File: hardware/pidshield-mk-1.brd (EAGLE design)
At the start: 43 x 52 mm, 32 parts, among them IC1 MAX31855, IC2 LM2931-3.3V, Q1 2N7000, Q2 2N7000, Q3 2N7000, Q4 2N7000, U1 ARDUINO_SHIELDINSIDER

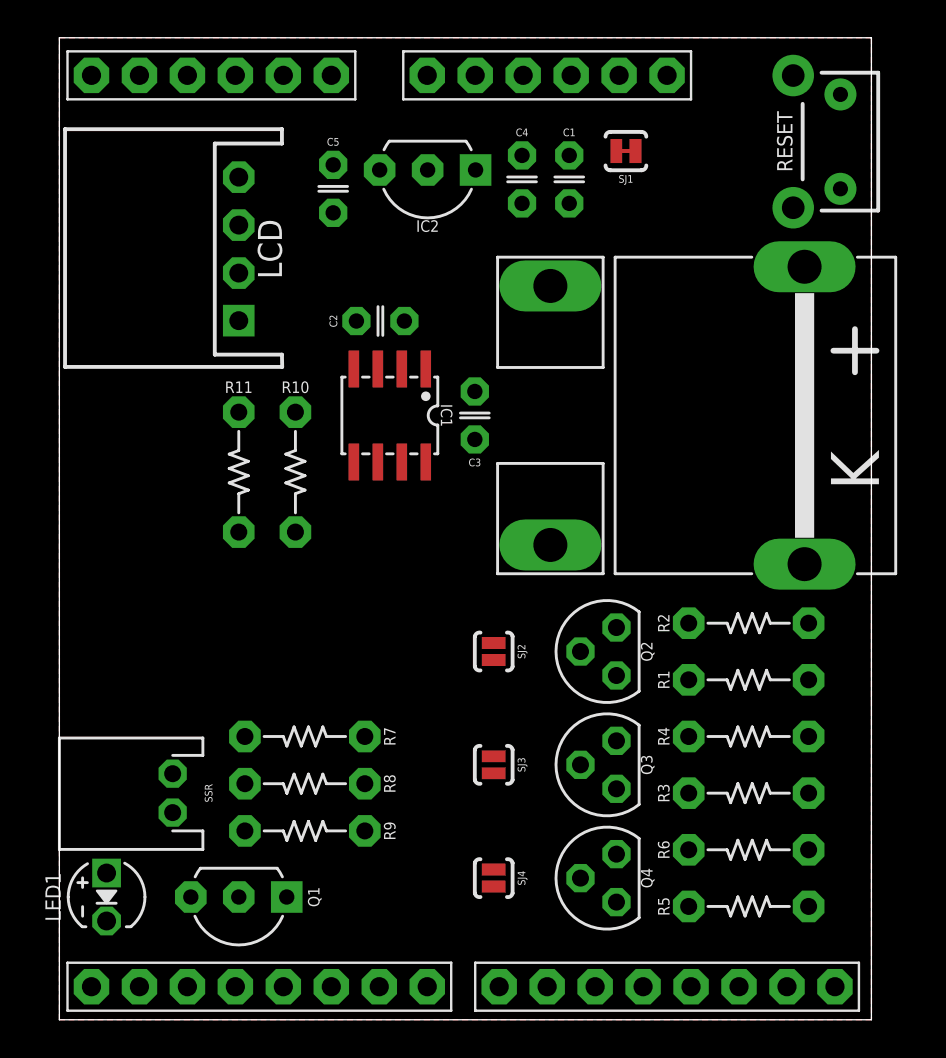
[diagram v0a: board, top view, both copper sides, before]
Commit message: think i've got the layout how i want it
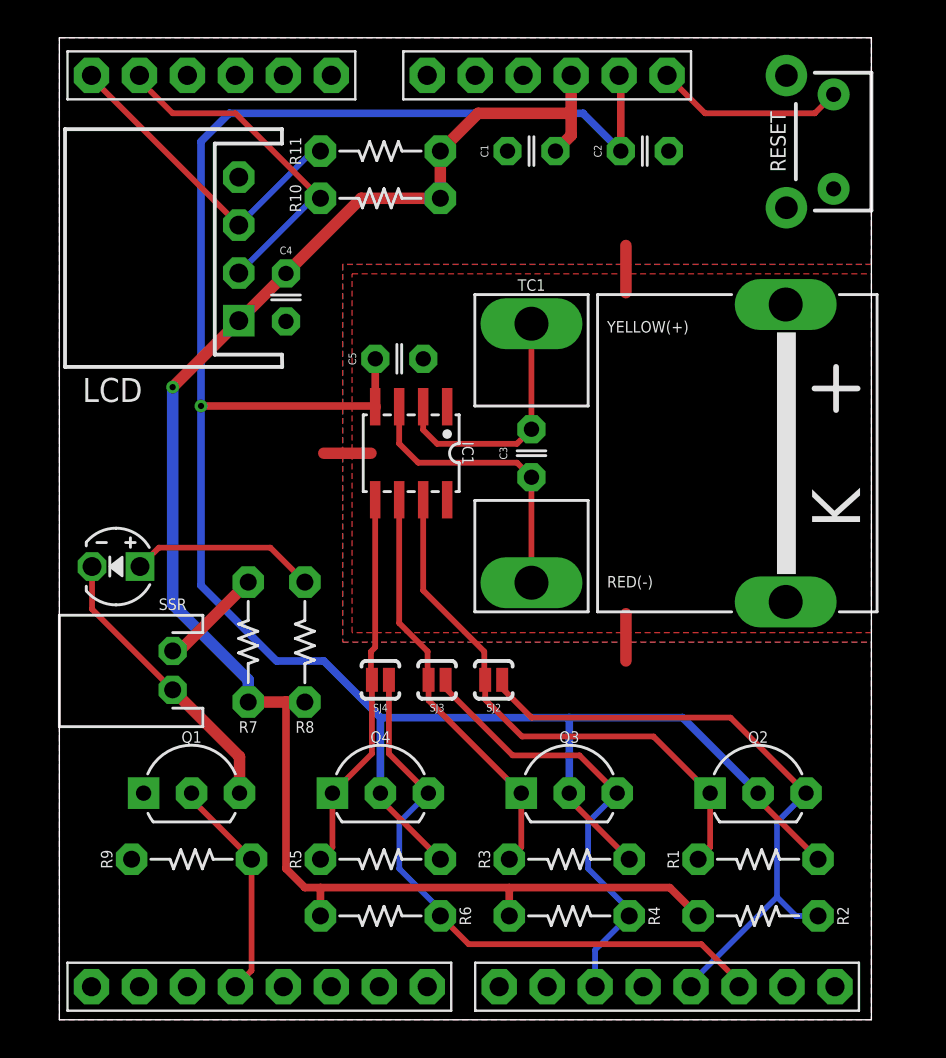
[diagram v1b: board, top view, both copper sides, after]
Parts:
- removed IC2: LM2931-3.3V, A_butts:TO-92-AMMO
- removed SJ1: JUMPER-PAD-2-NC_BY_TRACE, A_butts:PAD-JUMPER-2-NC_BY_TRACE_YES_SILK
- C1, C2: value 0.1uF -> 1uF
- C3: value 0.1uF -> 0.01uF
- C4, C5: value 1uF -> 0.1uF
- Q2, Q3, Q4: device A_butts:TO-92 -> A_butts:TO-92-AMMO
- TC1: value THERMOCOUPLE-CONNECTORMINI-PCB -> PCC-SMP-K
- moved R6 19.8 mm to (17.0, 5.50), turned to 180 degrees
- moved R5 19.7 mm to (17.0, 8.50)
- moved R11 18.6 mm to (17.0, 46.0), turned to 0 degrees
- moved LED1 17.5 mm to (3.00, 24.0), turned to 180 degrees
- moved C2 16.6 mm to (31.0, 46.0)
- moved R2 15.5 mm to (37.0, 5.50), turned to 180 degrees
- moved R10 15.2 mm to (17.0, 43.5), turned to 0 degrees
- moved C4 14.0 mm to (12.0, 38.2)
- moved R4 13.4 mm to (27.0, 5.50), turned to 180 degrees
- moved Q4 12.8 mm to (17.0, 12.0), turned to 0 degrees
- moved SJ4 12.1 mm to (17.0, 18.0), turned to 180 degrees
- moved Q2 11.0 mm to (37.0, 12.0), turned to 0 degrees
- moved R3 10.1 mm to (27.0, 8.50)
- moved C5 9.66 mm to (18.0, 35.0), turned to 0 degrees
- moved R1 9.51 mm to (37.0, 8.50)
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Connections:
- removed net N$1: SJ1.2, U1.3.3V
- net 3.3V: now also U1.3.3V; no longer IC2.3, SJ1.1
- net 5V: now also C1.2; no longer C1.1, IC2.1
- net GND: now also C1.1, R9.P$1, RESET.1; no longer C1.2, IC2.2, R9.P$2, RESET.2
- net RESET: now also RESET.2; no longer RESET.1
- net SSR: now also R9.P$2; no longer R9.P$1
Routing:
- net 3.3V: track 0.00 -> 119.5 mm, vias 0 -> 1
- net 5V: track 0.00 -> 89.0 mm, vias 0 -> 1
- net MISO-HOST: track 0.00 -> 34.2 mm
- net SCK-HOST: track 0.00 -> 32.4 mm
- net MISO-3V3: track 0.00 -> 29.7 mm
- net CS-HOST: track 0.00 -> 24.4 mm
- net CS-3V3: track 0.00 -> 22.0 mm
- net SCK-3V3: track 0.00 -> 20.3 mm
- net SDA: track 0.00 -> 18.4 mm
- net SCL: track 0.00 -> 17.1 mm
- net YELLOW(+): track 0.00 -> 15.3 mm
- net N$3: track 0.00 -> 15.2 mm
- net RED(-): track 0.00 -> 13.2 mm
- net SSR: track 0.00 -> 11.9 mm
- net RESET: track 0.00 -> 10.1 mm
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- added copper zone on layer 16, net GND
